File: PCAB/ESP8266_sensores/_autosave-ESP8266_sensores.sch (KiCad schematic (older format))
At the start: 18 parts, among them J1 Screw_Terminal_01x03, J2 Screw_Terminal_01x03, J3 Screw_Terminal_01x03, J4 Screw_Terminal_01x02, K1 SANYOU_SRD_Form_C, K2 SANYOU_SRD_Form_C, Q1 2N3904, Q2 2N3904, SW1 SW_Push

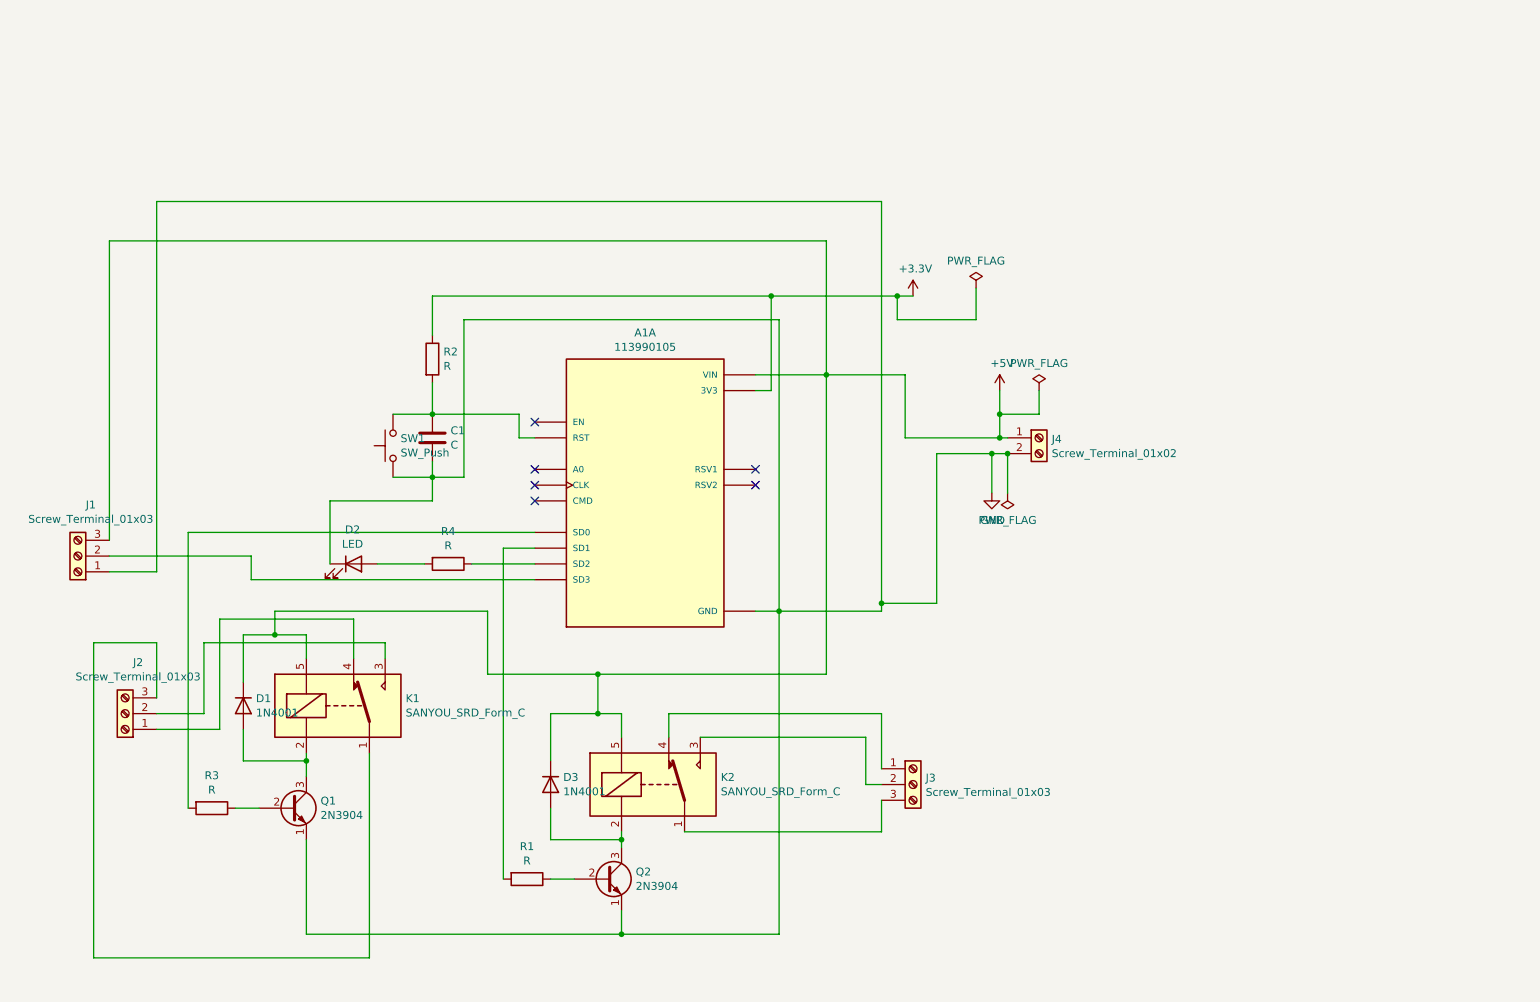
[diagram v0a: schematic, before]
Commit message: Agregando PCB2
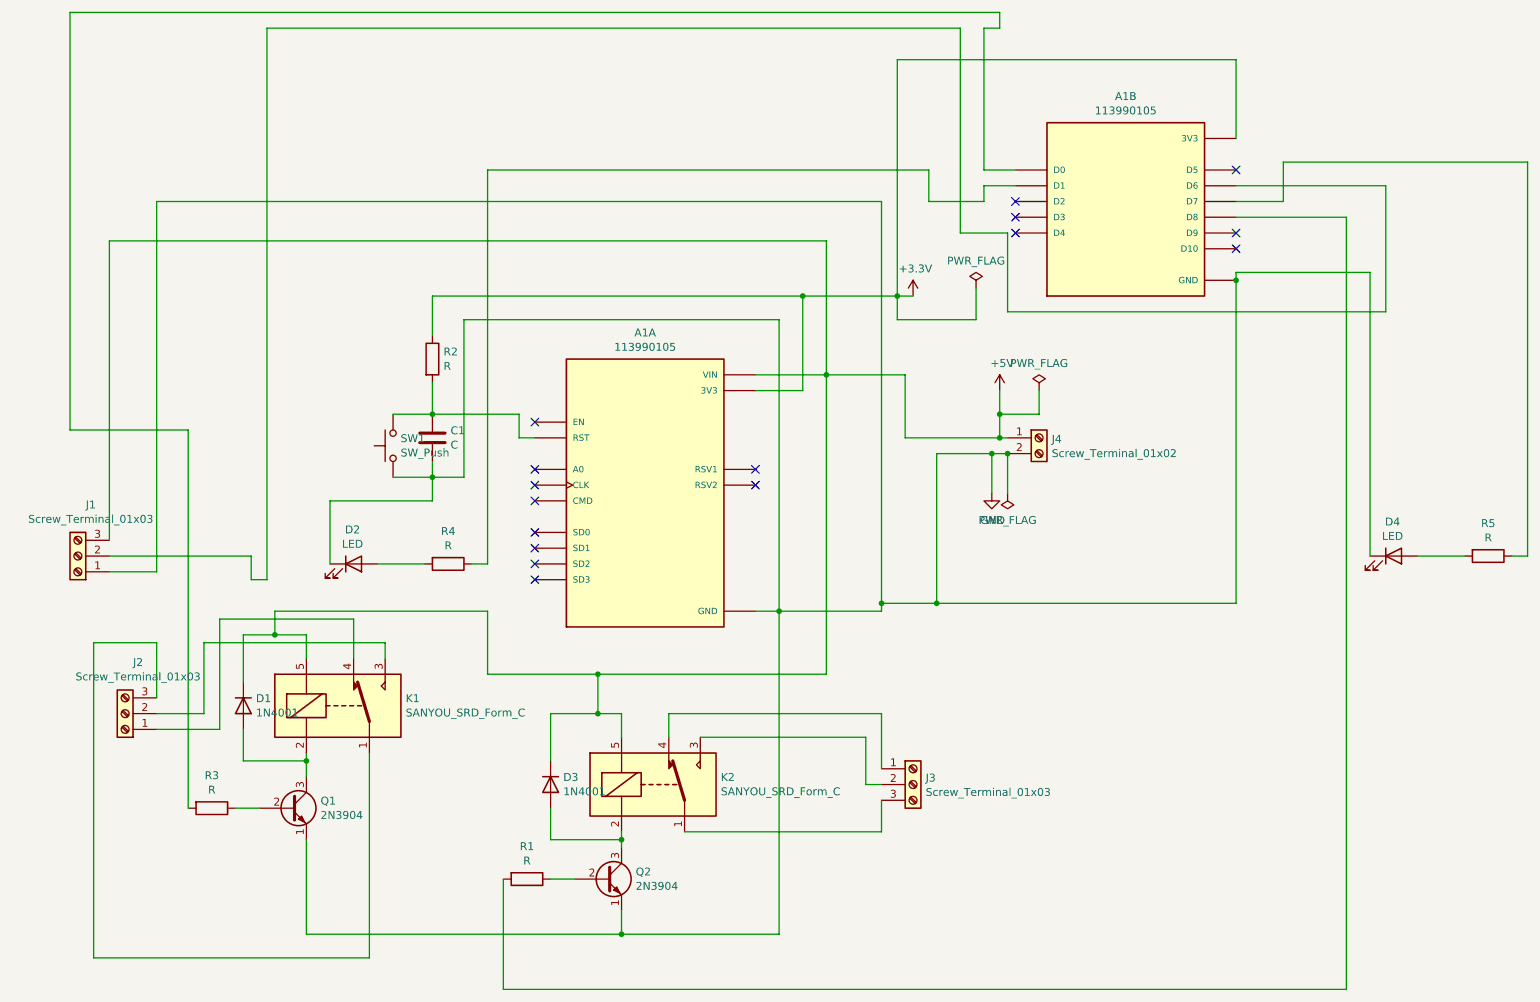
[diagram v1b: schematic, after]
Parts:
- added unit 2 of A1
- added D4: LED, LED_THT:LED_D5.0mm, symbol Device:LED
- added R5: R, Resistor_THT:R_Axial_DIN0207_L6.3mm_D2.5mm_P7.62mm_Horizontal, symbol Device:R
- A1: footprint kicad_libraries:SEEED_113990105 -> SEEED_113990105
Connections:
- net +3V3: now also A1.J2_15 (3V3), A1.J2_6 (3V3)
- net GND: now also A1.J2_14 (GND), A1.J2_7 (GND), D4.1 (K)
- net at J1.2 (Pin_2): now also A1.J2_9 (D6); no longer A1.J1_4 (SD3)
- net at R4.1: now also A1.J2_2 (D1); no longer A1.J1_5 (SD2)
- net at R1.2: now also A1.J2_11 (D8); no longer A1.J1_6 (SD1)
- net at R3.2: now also A1.J2_1 (D0); no longer A1.J1_8 (SD0)
- new net: A1.J2_10 (D7), R5.1
- new net: D4.2 (A), R5.2
- no-connect marks 6 -> 16
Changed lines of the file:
@@
 	3400 3750 3400 3650
-Wire Wire Line
-	5450 4600 5600 4600
 Wire Wire Line
 	5600 4600 5600 2750
@@
 	3600 3750 3400 3750
 Connection ~ 3400 3750
-$Comp
-L 113990105:113990105 A1
-U 1 1 635E7862
-P 4750 3800
-F 0 "A1" H 4750 4767 50  0000 C CNN
-F 1 "113990105" H 4750 4676 50  0000 C CNN
-F 2 "kicad_libraries:SEEED_113990105" H 4750 3800 50  0001 L BNN
-F 3 "" H 4750 3800 50  0001 L BNN
-F 4 "N/A" H 4750 3800 50  0001 L BNN "PARTREV"
-F 5 "Seeed" H 4750 3800 50  0001 L BNN "MANUFACTURER"
-F 6 "N/A" H 4750 3800 50  0001 L BNN "MAXIMUM_PACKAGE_HEIGHT"
-F 7 "Manufacturer Recommendations" H 4750 3800 50  0001 L BNN "STANDARD"
-	1    4750 3800
-	1    0    0    -1
-$EndComp
-Wire Wire Line
-	5550 3200 5550 2600
-Wire Wire Line
-	5550 2600 3400 2600
 Wire Wire Line
 	3400 3350 3950 3350
-Wire Wire Line
-	3950 3350 3950 3500
-Wire Wire Line
-	3950 3500 4050 3500
 $Comp
 L Transistor_BJT:2N3904 Q2
@@
 Connection ~ 4600 6650
 Wire Wire Line
-	5450 3100 5900 3100
-Wire Wire Line
 	5900 3100 5900 5000
 Wire Wire Line
@@
 	2400 4750 2600 4750
 Connection ~ 4450 5000
-Wire Wire Line
-	4050 4100 1850 4100
-Wire Wire Line
-	1850 4100 1850 5850
-Wire Wire Line
-	4050 4200 3850 4200
-Wire Wire Line
-	3850 4200 3850 6300
 $Comp
 L Device:LED D2
@@
 $EndComp
 Wire Wire Line
-	3650 4300 4050 4300
-Wire Wire Line
 	3050 4300 3350 4300
 Wire Wire Line
@@
 	1350 4250 2250 4250
 Wire Wire Line
-	2250 4250 2250 4400
-Wire Wire Line
-	2250 4400 4050 4400
-Wire Wire Line
 	5900 3100 5900 2250
 Wire Wire Line
@@
 Wire Wire Line
 	3400 2850 3400 2600
-Wire Wire Line
-	5450 3200 5550 3200
 $Comp
 L power:+3.3V #PWR0101
@@
 	1    0    0    -1
 $EndComp
-Wire Wire Line
-	5550 2600 6350 2600
-Connection ~ 5550 2600
 $Comp
 L power:PWR_FLAG #FLG0101
@@
 Wire Wire Line
 	6350 2600 6450 2600
+Wire Wire Line
+	3750 1800 3750 4300
+Wire Wire Line
+	3750 4300 3650 4300
+Wire Wire Line
+	2250 4250 2250 4400
+Wire Wire Line
+	6750 900  2350 900
+Wire Wire Line
+	2350 900  2350 4400
+Wire Wire Line
+	2350 4400 2250 4400
+Wire Wire Line
+	6900 900  7000 900
+Wire Wire Line
+	7000 900  7000 800
+Wire Wire Line
+	7000 800  1100 800
+Wire Wire Line
+	1100 800  1100 3450
+Wire Wire Line
+	1100 3450 1850 3450
+Wire Wire Line
+	1850 3450 1850 5850
+Wire Wire Line
+	9200 7000 3850 7000
+Wire Wire Line
+	3850 7000 3850 6300
+NoConn ~ 8500 1800
+NoConn ~ 8500 2200
+NoConn ~ 8500 2300
+$Comp
+L Device:LED D4
+U 1 1 6372CE72
+P 9500 4250
+F 0 "D4" H 9493 4467 50  0000 C CNN
+F 1 "LED" H 9493 4376 50  0000 C CNN
+F 2 "LED_THT:LED_D5.0mm" H 9500 4250 50  0001 C CNN
+F 3 "~" H 9500 4250 50  0001 C CNN
+	1    9500 4250
+	1    0    0    -1
+$EndComp
+$Comp
+L Device:R R5
+U 1 1 6372D13C
+P 10100 4250
+F 0 "R5" V 9893 4250 50  0000 C CNN
+F 1 "R" V 9984 4250 50  0000 C CNN
+F 2 "Resistor_THT:R_Axial_DIN0207_L6.3mm_D2.5mm_P7.62mm_Horizontal" V 10030 4250 50  0001 C CNN
+F 3 "~" H 10100 4250 50  0001 C CNN
+	1    10100 4250
+	0    1    1    0
+$EndComp
+Wire Wire Line
+	9650 4250 9950 4250
+Wire Wire Line
+	10350 1750 10350 4250
+Wire Wire Line
+	10350 4250 10250 4250
+NoConn ~ 4050 4100
+NoConn ~ 4050 4200
+NoConn ~ 4050 4300
+NoConn ~ 4050 4400
+Wire Wire Line
+	9350 2450 8500 2450
+Wire Wire Line
+	9350 2450 9350 4250
+Connection ~ 6600 4550
+Wire Wire Line
+	8500 4550 6600 4550
+Wire Wire Line
+	6350 1100 6350 2600
+Wire Wire Line
+	8500 1600 8500 1100
+Wire Wire Line
+	8500 1100 6350 1100
+Wire Wire Line
+	3400 2600 5750 2600
+$Comp
+L 113990105:113990105 A1
+U 1 1 637695E8
+P 4750 3800
+F 0 "A1" H 4750 4767 50  0000 C CNN
+F 1 "113990105" H 4750 4676 50  0000 C CNN
+F 2 "SEEED_113990105" H 4750 3800 50  0001 L BNN
+F 3 "" H 4750 3800 50  0001 L BNN
+F 4 "N/A" H 4750 3800 50  0001 L BNN "PARTREV"
+F 5 "Seeed" H 4750 3800 50  0001 L BNN "MANUFACTURER"
+F 6 "N/A" H 4750 3800 50  0001 L BNN "MAXIMUM_PACKAGE_HEIGHT"
+F 7 "Manufacturer Recommendations" H 4750 3800 50  0001 L BNN "STANDARD"
+	1    4750 3800
+	1    0    0    -1
+$EndComp
+Wire Wire Line
+	5450 3100 5900 3100
+Wire Wire Line
+	5450 3200 5750 3200
+Wire Wire Line
+	5750 3200 5750 2600
+Connection ~ 5750 2600
+Wire Wire Line
+	5750 2600 6350 2600
+Wire Wire Line
+	3950 3350 3950 3500
+Wire Wire Line
+	3950 3500 4050 3500
+Wire Wire Line
+	5450 4600 5600 4600
+Wire Wire Line
+	8500 2500 8500 4550
+Wire Wire Line
+	8500 2450 8500 2500
+Connection ~ 8500 2500
+$Comp
+L 113990105:113990105 A1
+U 2 1 636CAE54
+P 7800 2000
+F 0 "A1" H 7800 2667 50  0000 C CNN
+F 1 "113990105" H 7800 2576 50  0000 C CNN
+F 2 "SEEED_113990105" H 7800 2000 50  0001 L BNN
+F 3 "" H 7800 2000 50  0001 L BNN
+F 4 "N/A" H 7800 2000 50  0001 L BNN "PARTREV"
+F 5 "Seeed" H 7800 2000 50  0001 L BNN "MANUFACTURER"
+F 6 "N/A" H 7800 2000 50  0001 L BNN "MAXIMUM_PACKAGE_HEIGHT"
+F 7 "Manufacturer Recommendations" H 7800 2000 50  0001 L BNN "STANDARD"
+	2    7800 2000
+	1    0    0    -1
+$EndComp
+NoConn ~ 7100 2100
+Wire Wire Line
+	8500 2100 9200 2100
+Wire Wire Line
+	9200 2100 9200 7000
+Wire Wire Line
+	6900 1800 7100 1800
+Wire Wire Line
+	6900 900  6900 1800
+Wire Wire Line
+	3750 1800 6550 1800
+Wire Wire Line
+	6550 1800 6550 2000
+Wire Wire Line
+	6550 2000 6900 2000
+Wire Wire Line
+	6900 2000 6900 1900
+Wire Wire Line
+	6900 1900 7100 1900
+Wire Wire Line
+	6750 900  6750 2200
+Wire Wire Line
+	8800 1750 8800 2000
+Wire Wire Line
+	8800 2000 8500 2000
+Wire Wire Line
+	8800 1750 10350 1750
+NoConn ~ 7100 2000
+NoConn ~ 7100 2200
+Wire Wire Line
+	6750 2200 7050 2200
+Wire Wire Line
+	7050 2200 7050 2700
+Wire Wire Line
+	7050 2700 9450 2700
+Wire Wire Line
+	9450 2700 9450 1900
+Wire Wire Line
+	9450 1900 8500 1900
 $EndSCHEMATC
